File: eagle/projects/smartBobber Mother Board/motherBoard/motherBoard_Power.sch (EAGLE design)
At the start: 58 parts, among them J1 10118193-0001LF, J4 10118193-0001LF, U1 MCP7384XX, U2 MT3608, U3 LTC3531ES6-3_3, U4 MCP7384XX, U5 MT3608, U6 LTC3531ES6-3_3

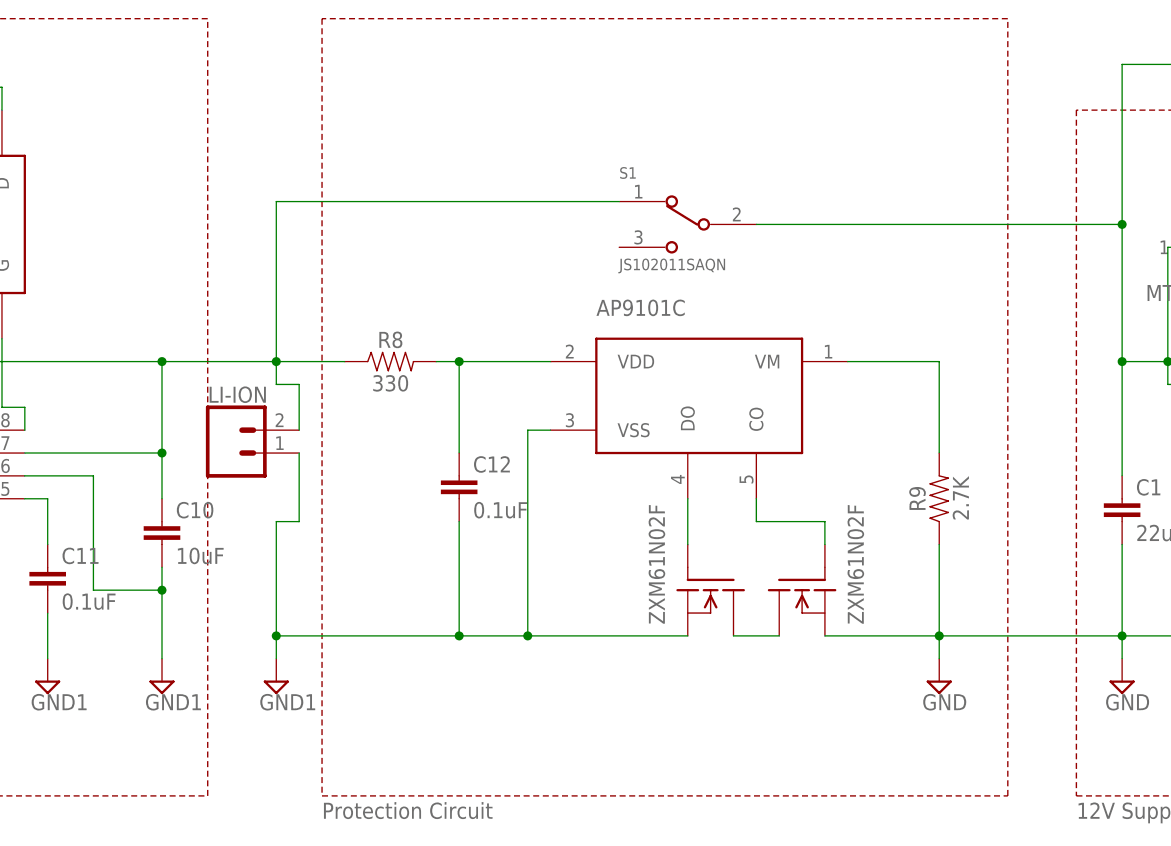
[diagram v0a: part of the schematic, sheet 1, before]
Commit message: Power-Schematic
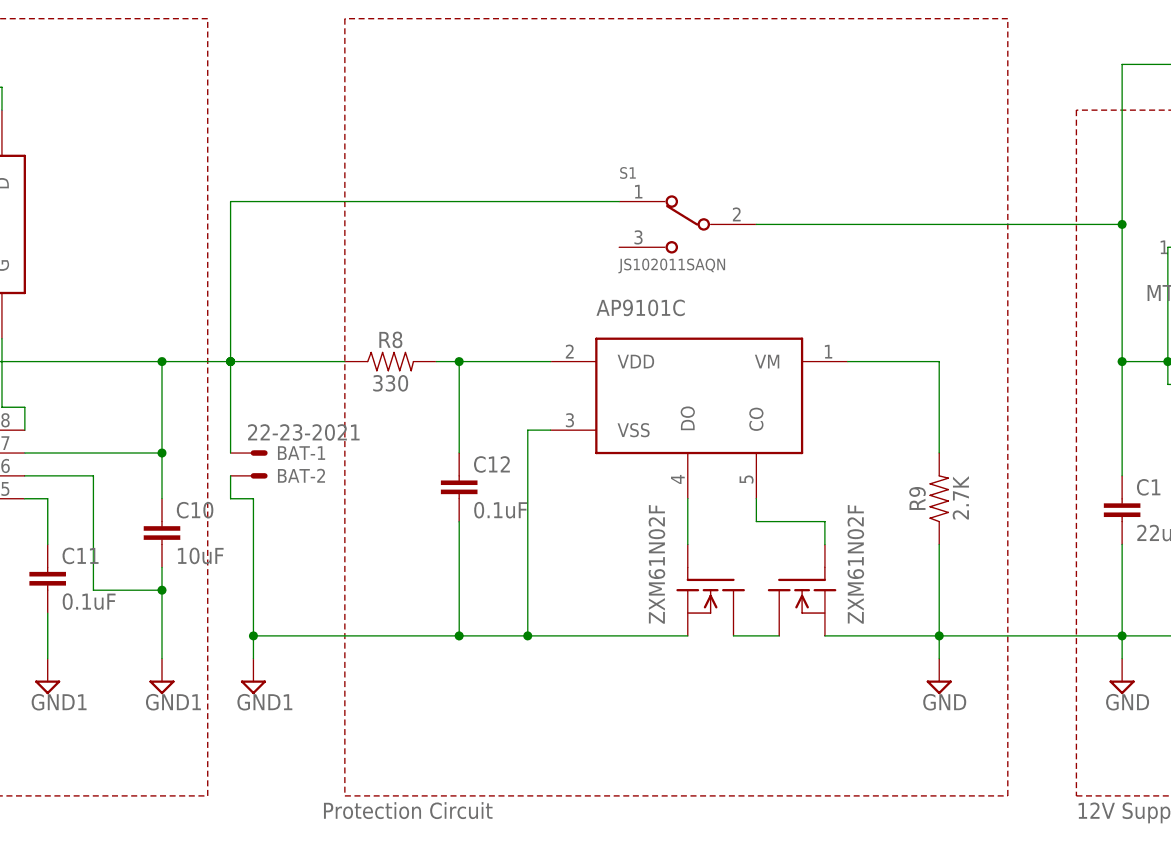
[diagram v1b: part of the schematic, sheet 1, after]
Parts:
- removed LI-ION: (no value), SparkFun-Connectors:CONN_02-JST-2-PTH-NO_SILK
- added BAT: 22-23-2021, con-molex:22-23-2021
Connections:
- net GND: now also BAT-2.S; no longer LI-ION.1
- net N$19: now also BAT-1.S; no longer LI-ION.2
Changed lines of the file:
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@@
 <part name="SUPPLY14" library="supply2" library_urn="urn:adsk.eagle:library:372" deviceset="GND" device=""/>
 <part name="SUPPLY15" library="supply2" library_urn="urn:adsk.eagle:library:372" deviceset="GND" device=""/>
-<part name="LI-ION" library="SparkFun-Connectors" deviceset="CONN_02" device="-JST-2-PTH-NO_SILK"/>
+<part name="BAT" library="con-molex" library_urn="urn:adsk.eagle:library:165" deviceset="22-23-2021" device=""/>
 </parts>
 <sheets>
@@
 <wire x1="20.32" y1="17.78" x2="20.32" y2="104.14" width="0.1524" layer="94" style="dashdot"/>
 <wire x1="20.32" y1="104.14" x2="-119.38" y2="104.14" width="0.1524" layer="94" style="dashdot"/>
-<wire x1="33.02" y1="104.14" x2="33.02" y2="17.78" width="0.1524" layer="94" style="dashdot"/>
-<wire x1="33.02" y1="17.78" x2="109.22" y2="17.78" width="0.1524" layer="94" style="dashdot"/>
+<wire x1="35.56" y1="104.14" x2="35.56" y2="17.78" width="0.1524" layer="94" style="dashdot"/>
+<wire x1="35.56" y1="17.78" x2="109.22" y2="17.78" width="0.1524" layer="94" style="dashdot"/>
 <wire x1="109.22" y1="17.78" x2="109.22" y2="104.14" width="0.1524" layer="94" style="dashdot"/>
-<wire x1="109.22" y1="104.14" x2="33.02" y2="104.14" width="0.1524" layer="94" style="dashdot"/>
+<wire x1="109.22" y1="104.14" x2="35.56" y2="104.14" width="0.1524" layer="94" style="dashdot"/>
 <wire x1="116.84" y1="93.98" x2="116.84" y2="17.78" width="0.1524" layer="94" style="dashdot"/>
 <wire x1="116.84" y1="17.78" x2="198.12" y2="17.78" width="0.1524" layer="94" style="dashdot"/>
@@
 <attribute name="VALUE" x="13.335" y="27.305" size="1.778" layer="96"/>
 </instance>
-<instance part="SUPPLY5" gate="GND" x="27.94" y="30.48" smashed="yes">
-<attribute name="VALUE" x="26.035" y="27.305" size="1.778" layer="96"/>
+<instance part="SUPPLY5" gate="GND" x="25.4" y="30.48" smashed="yes">
+<attribute name="VALUE" x="23.495" y="27.305" size="1.778" layer="96"/>
 </instance>
 <instance part="U$4" gate="G$1" x="76.2" y="63.5" smashed="yes"/>
@@
 <attribute name="VALUE" x="168.275" y="27.305" size="1.778" layer="96"/>
 </instance>
-<instance part="LI-ION" gate="G$1" x="22.86" y="55.88" smashed="yes">
-<attribute name="VALUE" x="20.32" y="51.054" size="1.778" layer="96" font="vector"/>
-<attribute name="NAME" x="20.32" y="61.468" size="1.778" layer="95" font="vector"/>
+<instance part="BAT" gate="-1" x="25.4" y="55.88" smashed="yes">
+<attribute name="NAME" x="27.94" y="55.118" size="1.524" layer="95"/>
+<attribute name="VALUE" x="24.638" y="57.277" size="1.778" layer="96"/>
+</instance>
+<instance part="BAT" gate="-2" x="25.4" y="53.34" smashed="yes">
+<attribute name="NAME" x="27.94" y="52.578" size="1.524" layer="95"/>
 </instance>
 </instances>
@@
 <pinref part="SUPPLY5" gate="GND" pin="GND"/>
 <pinref part="U$5" gate="G$1" pin="S"/>
-<wire x1="27.94" y1="35.56" x2="27.94" y2="33.02" width="0.1524" layer="91"/>
-<wire x1="27.94" y1="35.56" x2="48.26" y2="35.56" width="0.1524" layer="91"/>
+<wire x1="25.4" y1="35.56" x2="25.4" y2="33.02" width="0.1524" layer="91"/>
+<wire x1="25.4" y1="35.56" x2="48.26" y2="35.56" width="0.1524" layer="91"/>
 <wire x1="48.26" y1="35.56" x2="55.88" y2="35.56" width="0.1524" layer="91"/>
 <wire x1="55.88" y1="35.56" x2="73.66" y2="35.56" width="0.1524" layer="91"/>
@@
 <wire x1="48.26" y1="48.26" x2="48.26" y2="35.56" width="0.1524" layer="91"/>
 <junction x="48.26" y="35.56"/>
-<wire x1="27.94" y1="35.56" x2="27.94" y2="48.26" width="0.1524" layer="91"/>
-<junction x="27.94" y="35.56"/>
-<wire x1="27.94" y1="48.26" x2="30.48" y2="48.26" width="0.1524" layer="91"/>
-<pinref part="LI-ION" gate="G$1" pin="1"/>
-<wire x1="30.48" y1="48.26" x2="30.48" y2="55.88" width="0.1524" layer="91"/>
+<wire x1="25.4" y1="35.56" x2="25.4" y2="50.8" width="0.1524" layer="91"/>
+<junction x="25.4" y="35.56"/>
+<wire x1="25.4" y1="50.8" x2="22.86" y2="50.8" width="0.1524" layer="91"/>
+<pinref part="BAT" gate="-2" pin="S"/>
+<wire x1="22.86" y1="50.8" x2="22.86" y2="53.34" width="0.1524" layer="91"/>
 </segment>
 <segment>
@@
 <wire x1="-7.62" y1="68.58" x2="-7.62" y2="66.04" width="0.1524" layer="91"/>
 <wire x1="-7.62" y1="66.04" x2="15.24" y2="66.04" width="0.1524" layer="91"/>
-<junction x="27.94" y="66.04"/>
+<junction x="22.86" y="66.04"/>
 <pinref part="S1" gate="G$1" pin="1"/>
-<wire x1="15.24" y1="66.04" x2="27.94" y2="66.04" width="0.1524" layer="91"/>
-<wire x1="27.94" y1="66.04" x2="27.94" y2="83.82" width="0.1524" layer="91"/>
-<wire x1="27.94" y1="83.82" x2="66.04" y2="83.82" width="0.1524" layer="91"/>
+<wire x1="15.24" y1="66.04" x2="22.86" y2="66.04" width="0.1524" layer="91"/>
+<wire x1="22.86" y1="66.04" x2="22.86" y2="83.82" width="0.1524" layer="91"/>
+<wire x1="22.86" y1="83.82" x2="66.04" y2="83.82" width="0.1524" layer="91"/>
 <pinref part="R8" gate="G$1" pin="1"/>
-<wire x1="27.94" y1="66.04" x2="35.56" y2="66.04" width="0.1524" layer="91"/>
+<wire x1="22.86" y1="66.04" x2="35.56" y2="66.04" width="0.1524" layer="91"/>
 <pinref part="U1" gate="G$1" pin="VBAT"/>
 <wire x1="0" y1="55.88" x2="15.24" y2="55.88" width="0.1524" layer="91"/>
@@
 <junction x="15.24" y="66.04"/>
 <junction x="15.24" y="55.88"/>
-<pinref part="LI-ION" gate="G$1" pin="2"/>
-<wire x1="30.48" y1="58.42" x2="30.48" y2="63.5" width="0.1524" layer="91"/>
-<wire x1="30.48" y1="63.5" x2="27.94" y2="63.5" width="0.1524" layer="91"/>
-<wire x1="27.94" y1="63.5" x2="27.94" y2="66.04" width="0.1524" layer="91"/>
-</segment>
-</net>
+<pinref part="BAT" gate="-1" pin="S"/>
+<wire x1="22.86" y1="66.04" x2="22.86" y2="55.88" width="0.1524" layer="91"/>
+<junction x="22.86" y="66.04"/>
+</segment>
+</net>
